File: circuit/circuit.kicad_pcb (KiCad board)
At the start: 2 copper layers, 60 parts, among them P1 USB_A, U1 MIC5219BM5_SOT23-5

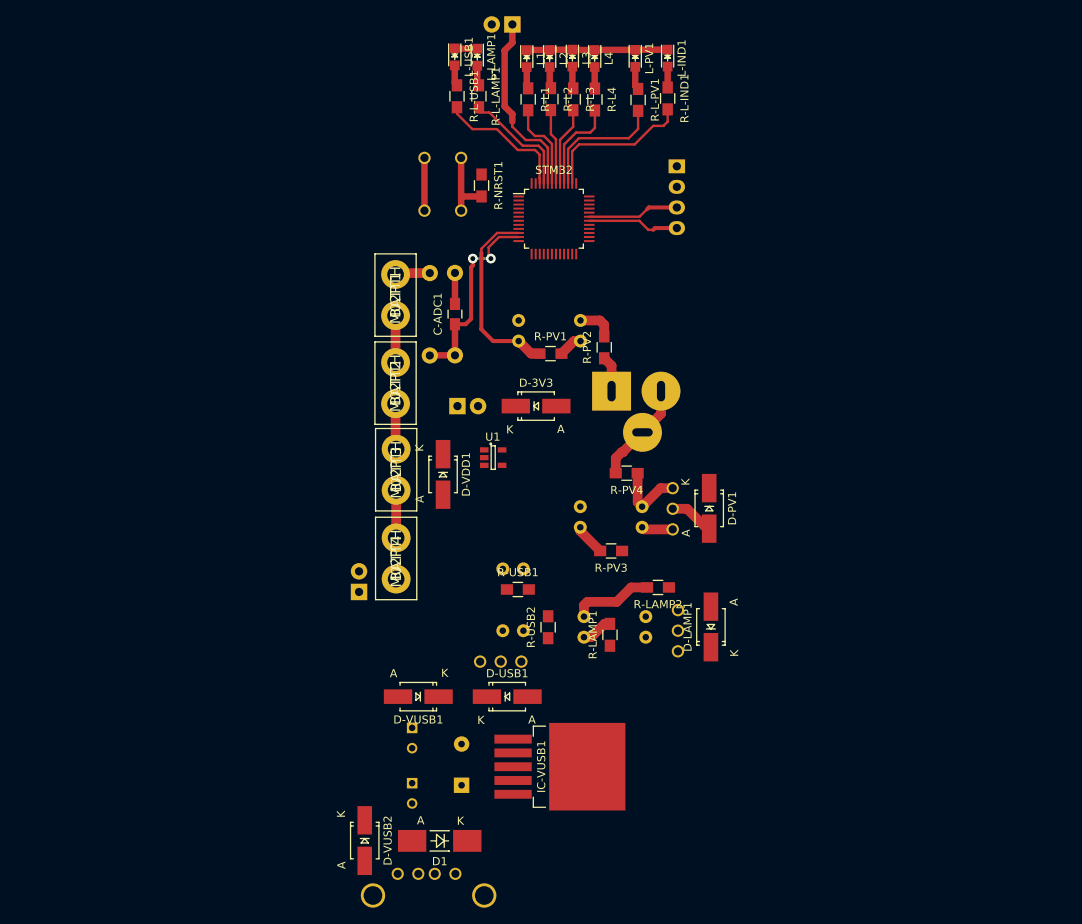
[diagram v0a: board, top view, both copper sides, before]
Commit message: circuit building
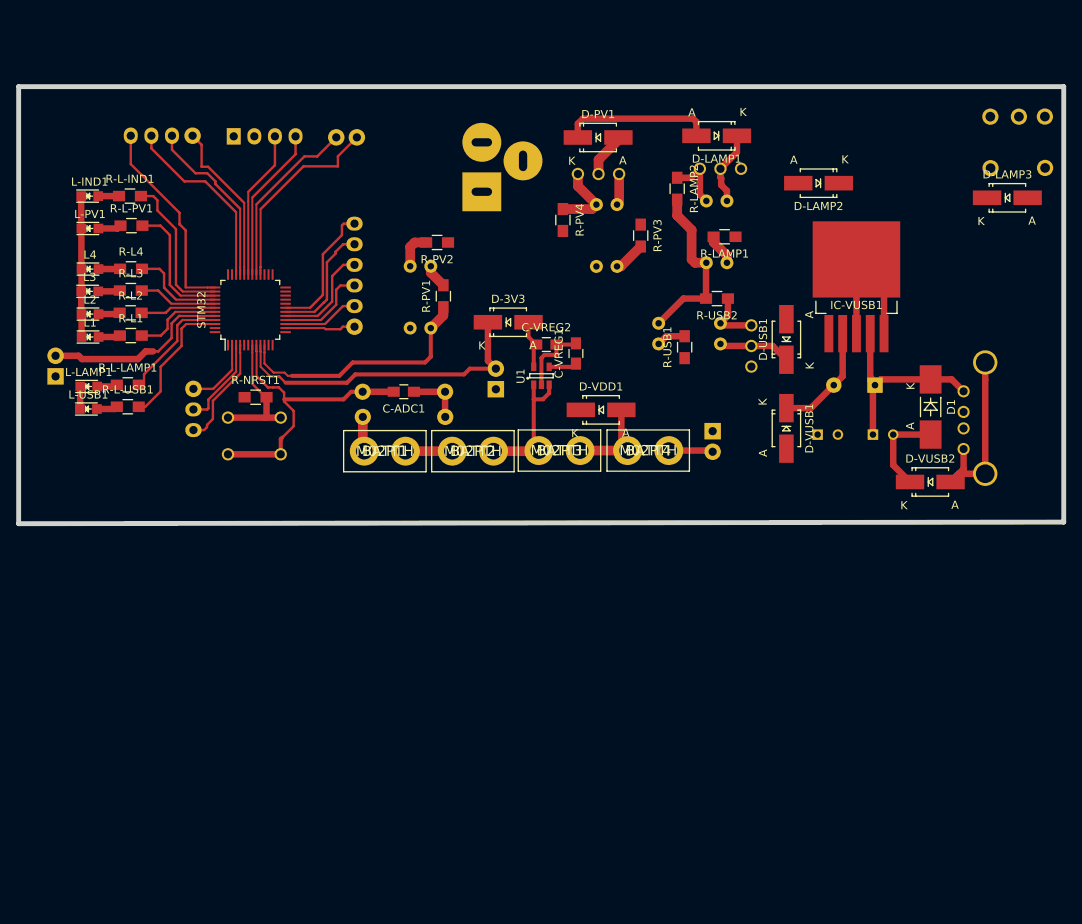
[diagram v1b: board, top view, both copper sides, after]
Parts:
- added C-VREG1: C, Capacitors_SMD:C_0805_HandSoldering, F.Cu at (155.3, 89.0)
- added C-VREG2: C, Capacitors_SMD:C_0805_HandSoldering, F.Cu at (151.7, 87.9)
- added D-LAMP2: D, Diodes_SMD:SMA_Handsoldering, F.Cu at (185.2, 68.0)
- added D-LAMP3: D_Schottky, Diodes_SMD:SMA_Handsoldering, F.Cu at (208.5, 69.8)
- added J1: audio-jack, audio-lamp:JACK_LAPAN, B.Cu at (212.7, 56.3)
- added P2: CONN_01X04, Pin_Headers:Pin_Header_Straight_1x04, B.Cu at (108.1, 62.2)
- added PIN1: CONN_01X03, Pin_Headers:Pin_Header_Straight_1x03, B.Cu at (108.2, 93.4)
- added PIN2: CONN_01X06, Pin_Headers:Pin_Header_Straight_1x06, B.Cu at (128.0, 85.7)
- added PIN3: CONN_01X02, Pin_Headers:Pin_Header_Straight_1x02, B.Cu at (128.3, 62.4)
- moved P1 86.4 mm to (203.1, 93.7), turned to 270 degrees
- moved D-VUSB2 82.5 mm to (199.0, 104.9), turned to 0 degrees
- moved D1 80.8 mm to (199.0, 95.6), turned to 270 degrees
- moved L-IND1 73.2 mm to (95.4, 69.6), turned to 0 degrees
- moved C_VUSB2 71.2 mm to (191.9, 99.0), turned to 0 degrees
- moved P-BOOT1 71.1 mm to (91.2, 91.8), turned to 0 degrees
- moved L-PV1 70.4 mm to (95.4, 73.6), turned to 0 degrees
- moved IC-VUSB1 68.1 mm to (189.9, 86.6), turned to 90 degrees
- moved L4 67.4 mm to (95.4, 78.6), turned to 0 degrees
- moved R-L-IND1 67.4 mm to (100.3, 69.6), turned to 0 degrees
- moved L-VUSB1 67.3 mm to (189.6, 92.9), turned to 180 degrees
- moved L3 66.1 mm to (95.4, 81.4), turned to 0 degrees
- moved L2 64.8 mm to (95.4, 84.2), turned to 0 degrees
- moved R-L-PV1 64.3 mm to (100.5, 73.3), turned to 0 degrees
- moved L1 63.8 mm to (95.4, 87.0), turned to 0 degrees
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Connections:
- P-BOOT1 pad 1: /BOOT0 -> VDD
- P-BOOT1 pad 2: VDD -> /BOOT0
- STM32 pad 1: Net-(STM32-Pad1) -> VDD
- STM32 pad 14: Net-(STM32-Pad14) -> /AIN4
- STM32 pad 15: Net-(STM32-Pad15) -> /AIN5
- STM32 pad 16: Net-(STM32-Pad16) -> /AIN6
- STM32 pad 17: Net-(STM32-Pad17) -> /AIN7
- STM32 pad 18: Net-(STM32-Pad18) -> /AIN8
- STM32 pad 19: Net-(STM32-Pad19) -> /AIN9
- STM32 pad 2: Net-(STM32-Pad2) -> /PC13
- STM32 pad 28: Net-(STM32-Pad28) -> /PB15
- STM32 pad 29: Net-(STM32-Pad29) -> /PA8
- STM32 pad 3: Net-(STM32-Pad3) -> /PC14
- STM32 pad 32: Net-(STM32-Pad32) -> /PA11
- STM32 pad 33: Net-(STM32-Pad33) -> /PA12
- STM32 pad 34: Net-(STM32-Pad34) -> /PA13
- STM32 pad 37: Net-(STM32-Pad37) -> /PA14
- STM32 pad 4: Net-(STM32-Pad4) -> /PC15
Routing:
- net GND: track 43.6 -> 122.0 mm
- net +3V3: track 0.00 -> 39.3 mm
- net Net-(C_VUSB2-Pad1): track 0.00 -> 25.6 mm
- net /PA14: track 0.00 -> 25.1 mm
- net /PB15: track 0.00 -> 24.3 mm
- net /ADC_USB: track 0.00 -> 23.1 mm
- net /PA13: track 0.00 -> 22.9 mm
- net /PA8: track 0.00 -> 21.9 mm
- net /PA12: track 0.00 -> 21.4 mm
- net /PA11: track 0.00 -> 20.2 mm
- net +15V: track 4.30 -> 22.7 mm
- net /ADC_BATT: track 24.7 -> 6.94 mm, vias 2 -> 0
- net /AIN9: track 0.00 -> 16.4 mm
- net /AIN8: track 0.00 -> 14.8 mm
- net Net-(D-VUSB1-Pad1): track 0.00 -> 13.8 mm
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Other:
- board outline added: 128.8 x 53.9 mm
